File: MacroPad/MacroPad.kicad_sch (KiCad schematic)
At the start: 1 part

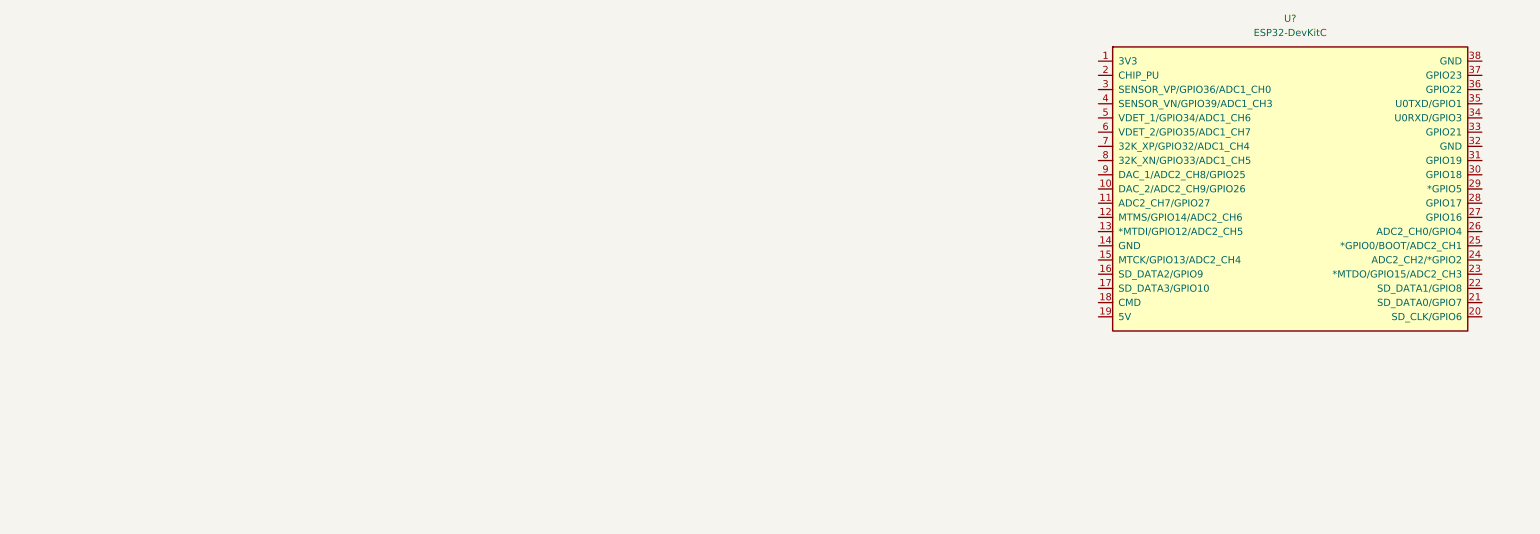
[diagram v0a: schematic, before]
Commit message: RGB LED Circuit
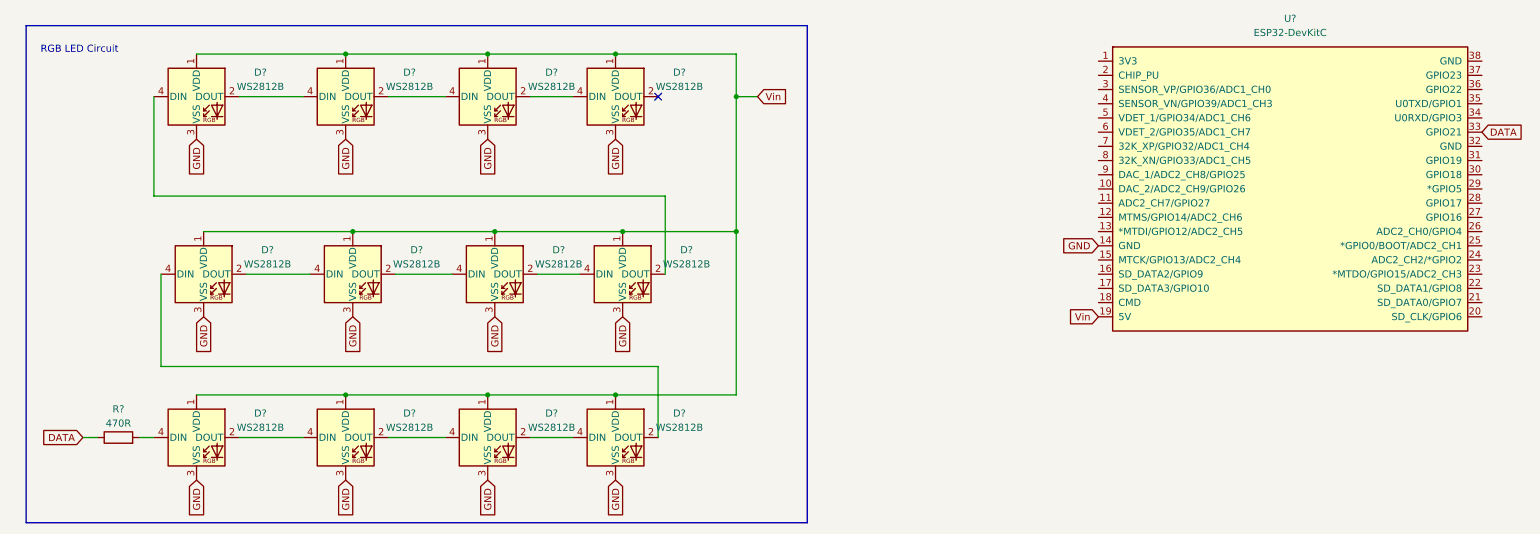
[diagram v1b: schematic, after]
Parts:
- added D? (x12): WS2812B, LED_SMD:LED_WS2812B_PLCC4_5.0x5.0mm_P3.2mm, symbol LED:WS2812B
- added R?: 470R, symbol Device:R
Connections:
- net GND: now reaches U?.14 (GND)
- net GND: now also D?.3 (VSS), D?.3 (VSS), D?.3 (VSS), D?.3 (VSS), D?.3 (VSS), D?.3 (VSS), D?.3 (VSS), D?.3 (VSS), D?.3 (VSS), D?.3 (VSS), D?.3 (VSS), D?.3 (VSS)
- net Vin: now reaches U?.19 (5V)
- net Vin: now also D?.1 (VDD), D?.1 (VDD), D?.1 (VDD), D?.1 (VDD), D?.1 (VDD), D?.1 (VDD), D?.1 (VDD), D?.1 (VDD), D?.1 (VDD), D?.1 (VDD), D?.1 (VDD), D?.1 (VDD)
- net DATA: now reaches U?.33 (GPIO21)
- net DATA: now also R?.1
- new net: D?.2 (DOUT), D?.4 (DIN) (x11)
- new net: D?.4 (DIN), R?.2
- no-connect marks 0 -> 1
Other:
- note added: "RGB LED Circuit"
